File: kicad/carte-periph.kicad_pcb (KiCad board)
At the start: 2 copper layers, 80 x 72.4 mm, 30 parts, among them J1 PDB, J2 PWR_IN, J3 PROG, J8 I2C, J9 I2C, U1 Conn_periph, U2 PIC24FJ128GA104, Y1 10MHz

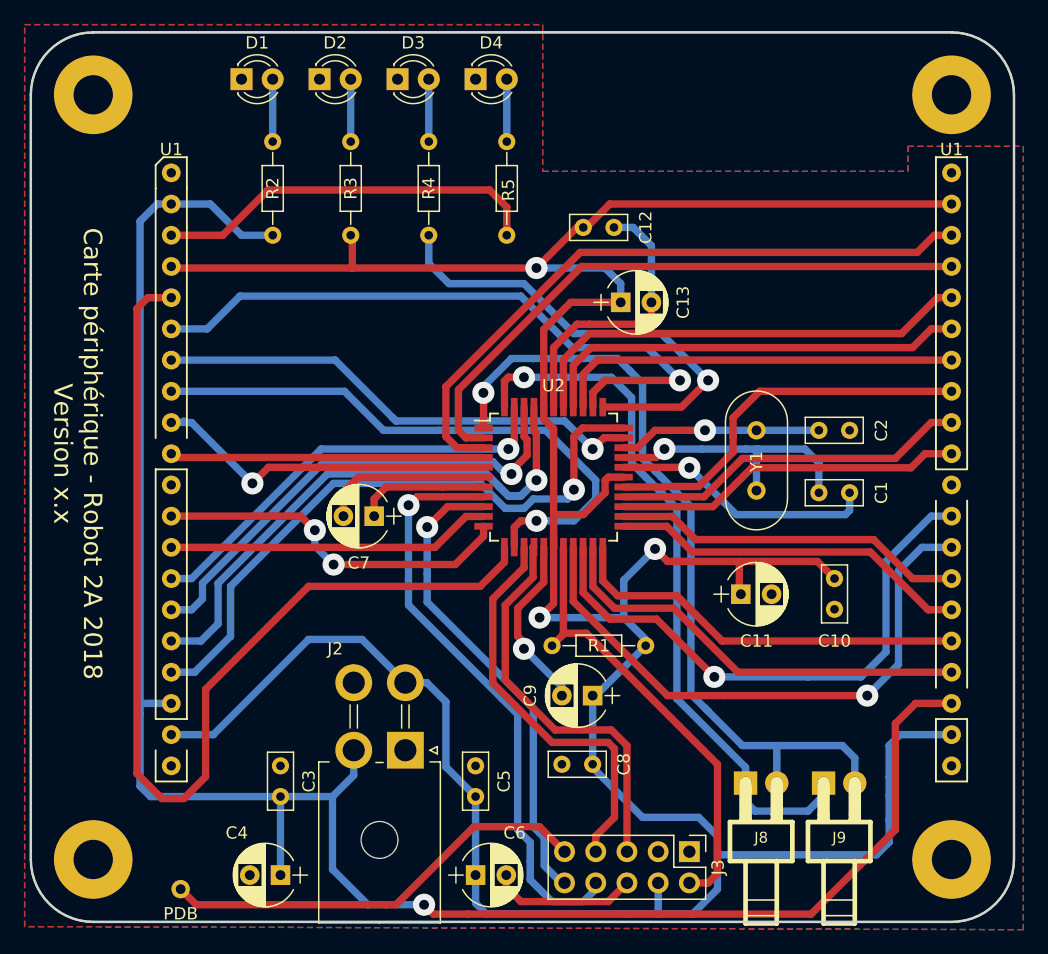
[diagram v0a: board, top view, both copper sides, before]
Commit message: Validation carte, à passer en release
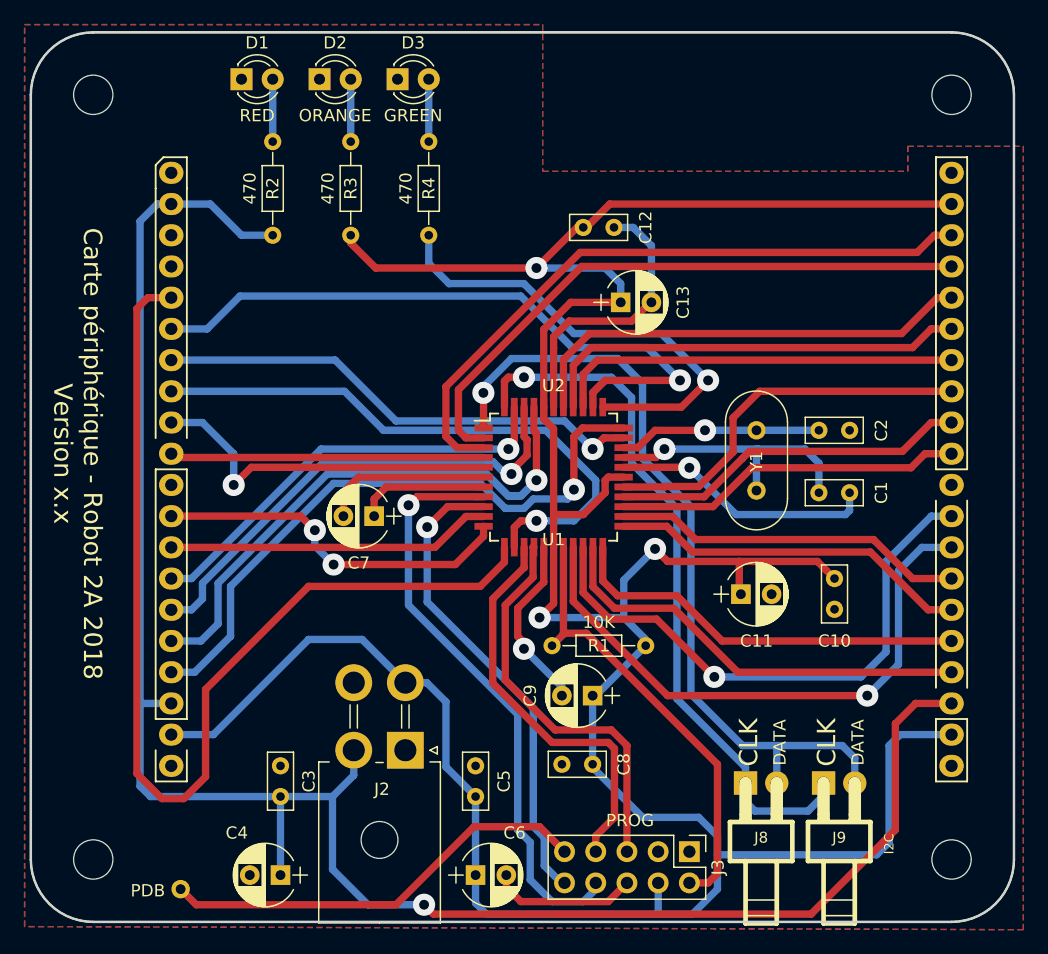
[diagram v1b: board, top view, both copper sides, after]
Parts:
- removed D4: RED, LEDs:LED_D3.0mm
- removed R5: 470, Resistors_THT:R_Axial_DIN0204_L3.6mm_D1.6mm_P7.62mm_Horizontal
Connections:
- U1 pad L1: Net-(R5-Pad2) -> (no net)
- U1 pad V34: +3V3 -> (no net)
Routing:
- net Net-(R5-Pad2): track 31.7 -> 0.00 mm
- net +3V3: track 277.8 -> 261.0 mm
- net Net-(D4-Pad2): track 5.08 -> 0.00 mm
- net /RC9: track 28.1 -> 29.6 mm
- net GND: track 85.9 -> 84.9 mm
- net /PDT: track 48.5 -> 48.0 mm
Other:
- board text added: "CLK"
- board text added: "DATA"
